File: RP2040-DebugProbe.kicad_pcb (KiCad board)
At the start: 4 copper layers, 59.7 x 31.1 mm, 70 parts, among them J1 CONN_MCU_JTAG, J10 CONN_USB, J2 CONN_MCU_UART, J3 CONN_DBG_COMB, J4 CONN_3V3_JUMPER, J7 CONN_DBG_JTAG, SW1 BOOTSEL, U1 W25Q128JVS, U2 RP2040, U3 74AUP1T17, U4 W25Q128JVEIQ, U5 AMS1117-3.3, U6 74AUP1T17, Y1 12MHz

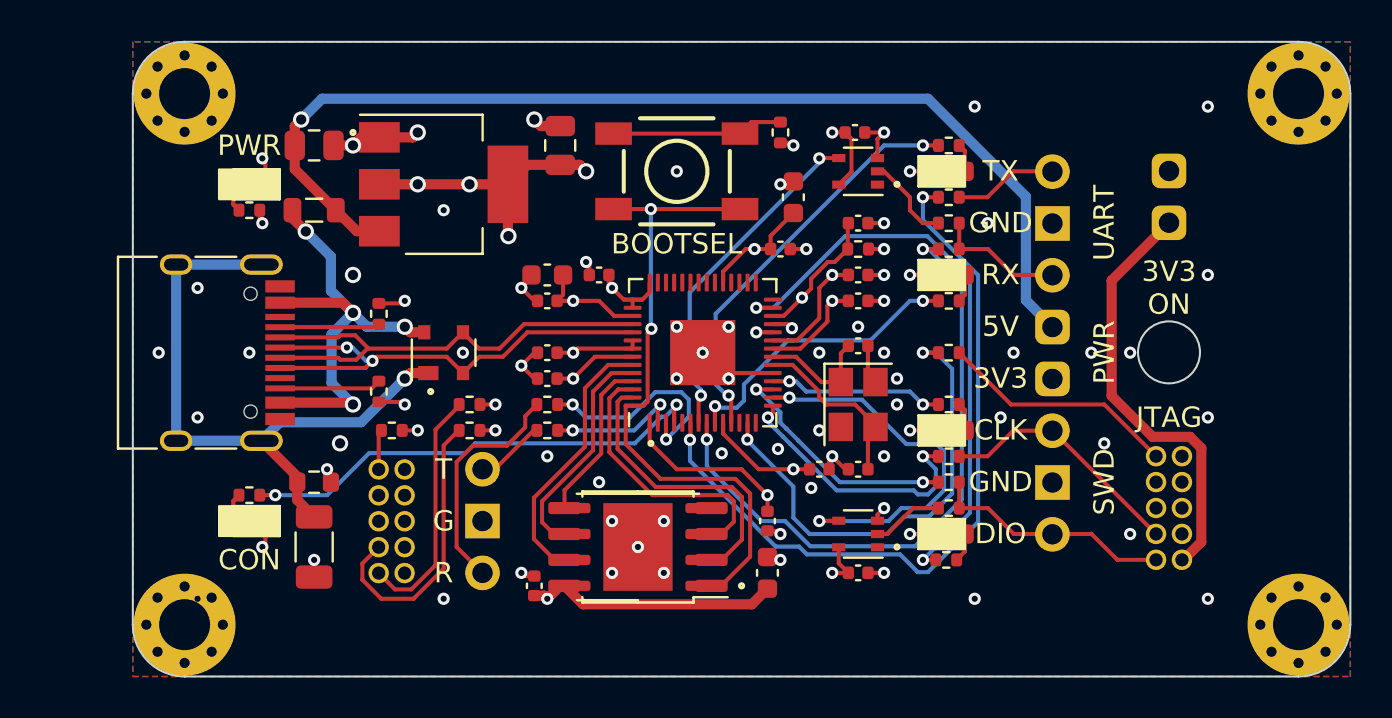
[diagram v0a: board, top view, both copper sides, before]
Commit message: tinyprogrammer
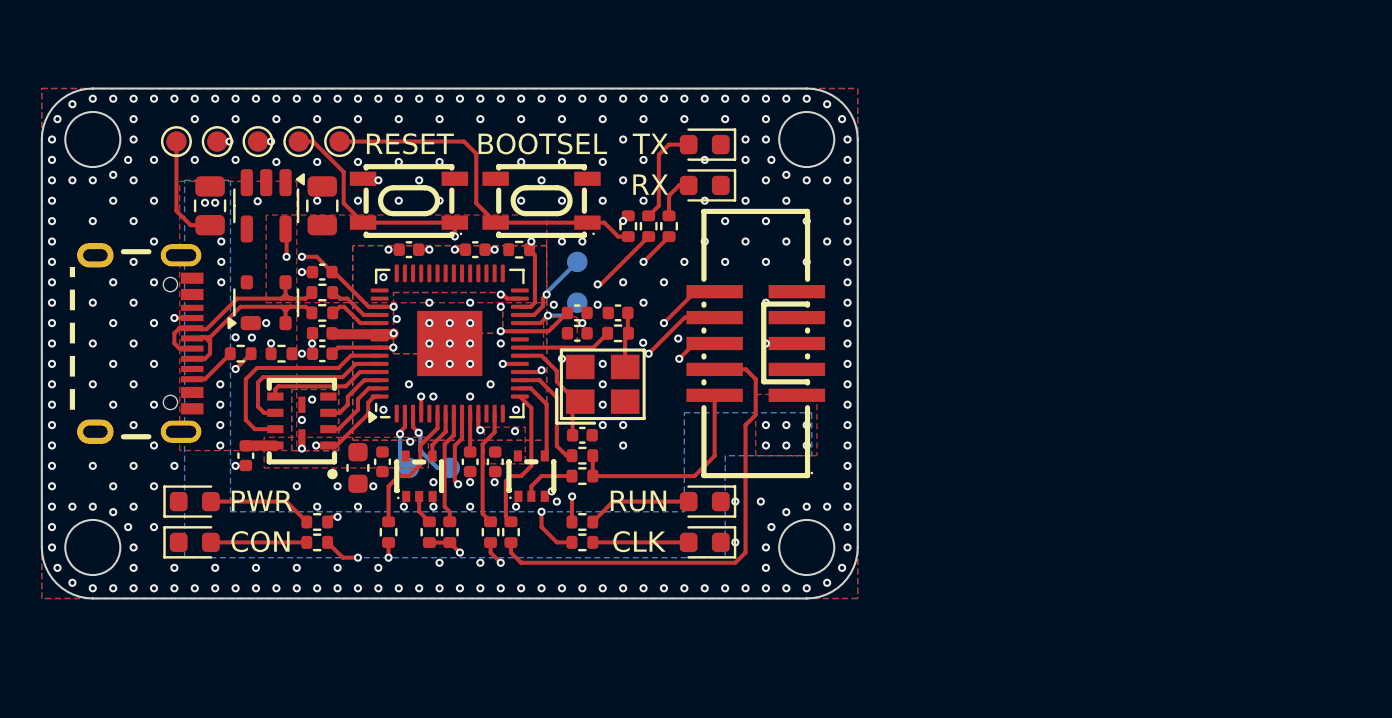
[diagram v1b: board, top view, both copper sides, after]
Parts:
- removed C1, C5: 2.2uF, Capacitor_SMD:C_0603_1608Metric
- removed C12, C13: 100nF, Capacitor_SMD:C_0402_1005Metric
- removed C21: 4.7nF 1kV, Capacitor_SMD:C_1206_3216Metric
- removed FB2: 100@100MHz, Inductor_SMD:L_0805_2012Metric
- removed H1, H2, H3, H4: MountingHole_Pad, MountingHole:MountingHole_2.5mm_Pad_Via
- removed J1: CONN_MCU_JTAG, Connector_PinHeader_1.27mm:PinHeader_2x05_P1.27mm_Vertical
- removed J2: CONN_MCU_UART, Connector_PinHeader_2.54mm:PinHeader_1x03_P2.54mm_Vertical
- removed J3: CONN_DBG_COMB, Connector_PinHeader_2.54mm:PinHeader_1x08_P2.54mm_Vertical
- removed J4: CONN_3V3_JUMPER, Connector_PinHeader_2.54mm:PinHeader_1x02_P2.54mm_Vertical
- removed J7: CONN_DBG_JTAG, Connector_PinHeader_1.27mm:PinHeader_2x05_P1.27mm_Vertical
- removed R20, R21, R22, R23: 100R, Resistor_SMD:R_0402_1005Metric
- removed R8: 10k, Resistor_SMD:R_0402_1005Metric
- removed SW1: BOOTSEL, PCM_4ms_Switch:Button_Tact_Sqkg
- added R24: 27R, Resistor_SMD:R_0402_1005Metric, F.Cu at (133.8, 106.0)
- added R25: 27R, Resistor_SMD:R_0402_1005Metric, F.Cu at (133.8, 105.0)
- added TP10: TestPoint, TestPoint:TestPoint_Pad_D1.0mm, B.Cu at (146.2, 103.5)
- added TP11: TestPoint, TestPoint:TestPoint_Pad_D1.0mm, B.Cu at (146.2, 105.5)
- added TP13: TestPoint, TestPoint:TestPoint_Pad_D1.0mm, F.Cu at (130.6, 97.6)
- added TP4: TestPoint, TestPoint:TestPoint_Pad_D1.0mm, F.Cu at (126.6, 97.6)
- added TP5: TestPoint, TestPoint:TestPoint_Pad_D1.0mm, F.Cu at (128.6, 97.6)
- added TP6: TestPoint, TestPoint:TestPoint_Pad_D1.0mm, F.Cu at (134.6, 97.6)
- added TP7: TestPoint, TestPoint:TestPoint_Pad_D1.0mm, F.Cu at (132.6, 97.6)
- added TP8: TestPoint, TestPoint:TestPoint_Pad_D1.0mm, B.Cu at (138.0, 113.6)
- added TP9: TestPoint, TestPoint:TestPoint_Pad_D1.0mm, B.Cu at (140.0, 113.6)
- added U7: HX_JN1_27-2X5_TP_H4_9, JLCPCB:IDC-SMD_10P-P1.27-3220-10-0300-00, F.Cu at (155.0, 107.5)
- added U8: TS-1089S-02526, JLCPCB:SW-SMD_4P-L4.2-W3.3-P2.15-LS5.1, F.Cu at (138.0, 100.5)
- C14, C15: value 10uF -> 22uF
- C19, C20: value 12pF -> 15pF
- J10: footprint Connector_USB:USB_C_Receptacle_HRO_TYPE-C-31-M-12 -> JLCPCB:USB-C-SMD_TYPE-C-6PIN-2MD-073
- R12: value 1M -> 1K; footprint Resistor_SMD:R_0603_1608Metric -> Resistor_SMD:R_0402_1005Metric
- R19: value 100R -> 10k
- U1: value W25Q128JVS -> AP2112K-3.3; footprint Package_SO:SOIC-8_5.23x5.23mm_P1.27mm -> Package_TO_SOT_SMD:SOT-23-5
- U3, U6: value 74AUP1T17 -> 74AUP1T17GWH; footprint Package_TO_SOT_SMD:SOT-353_SC-70-5 -> JLCPCB:TSSOP-5_L2.1-W1.3-P0.65-LS2.2-BR
- U4: value W25Q128JVEIQ -> W25Q64JVEIQ; footprint Package_SON:WSON-8-1EP_6x5mm_P1.27mm_EP3.4x4.3mm -> JLCPCB:USON-8_L4.0-W3.0-P0.80-BL_WINBOND_UU
- U5: value AMS1117-3.3 -> TS-1089S-02526; footprint Package_TO_SOT_SMD:SOT-223-3_TabPin2 -> JLCPCB:SW-SMD_4P-L4.2-W3.3-P2.15-LS5.1
- Y1: footprint Crystal:Crystal_SMD_3225-4Pin_3.2x2.5mm -> JLCPCB:CRYSTAL-SMD_4P-L3.2-W2.5-BL
- moved R15 32.0 mm to (137.0, 116.8), turned to 90 degrees
- moved R9 29.6 mm to (139.0, 116.8), turned to 90 degrees
- moved C17 28.2 mm to (136.7, 113.3), turned to -90 degrees
- moved R14 28.1 mm to (140.0, 116.8), turned to 90 degrees
- moved U3 26.2 mm to (138.5, 114.0), turned to -90 degrees
- moved U1 24.7 mm to (131.0, 100.8), turned to -90 degrees
- moved R18 24.1 mm to (142.0, 116.8), turned to 90 degrees
- moved R17 21.8 mm to (143.0, 116.8), turned to 90 degrees
- moved C16 20.7 mm to (135.5, 113.6), turned to -90 degrees
- moved C3 19.6 mm to (141.2, 102.9), turned to 0 degrees
- moved R4 19.2 mm to (146.5, 117.2)
- moved C4 18.2 mm to (138.0, 102.9)
- moved R13 18.0 mm to (146.5, 114.0)
- moved R16 18.0 mm to (146.5, 113.0)
- moved R5 17.9 mm to (146.5, 116.2)
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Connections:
- net Net-(D1-A) renamed /RLED_RX
- net Net-(D4-A) renamed /RLED_TX
- net Net-(D5-A) renamed /RLED_ACT
- net Net-(D6-A) renamed /RLED_CON
- net Net-(D7-A) renamed /RLED_RUN
- C15 pad 1: VUSB -> +5V
- C19 pad 1: XIN -> /XIN
- C20 pad 1: XOUT -> /ROUT
- D3 pad 1: SHIELD -> GND
- D3 pad 2: USB_DP -> USBC_DP
- D3 pad 3: USB_DN -> USBC_DN
- D3 pad 4: VBUS -> +5V
- R10 pad 1: Net-(J10-CC1) -> /CC1
- R11 pad 1: Net-(J10-CC2) -> /CC2
- R12 pad 1: SHIELD -> /XOUT
- R12 pad 2: GND -> /ROUT
- R19 pad 1: MCU_TX -> +3V3
- R19 pad 2: HOST_TX -> /RESET
- R7 pad 1: Net-(R7-Pad1) -> /QSPI_SS
- R7 pad 2: GND -> /BOOTSEL
- U1 pad 1: QSPI_SS -> +5V
- U1 pad 2: QSPI_SD1 -> GND
- U1 pad 3: QSPI_SD2 -> +5V
- U1 pad 4: GND -> unconnected-(U1-NC-Pad4)
- U1 pad 5: QSPI_SD0 -> +3V3
- U2 pad 2: MCU_TX -> /HOST_UART_TX
- U2 pad 20: XIN -> /XIN
- U2 pad 21: XOUT -> /XOUT
- U2 pad 24: MCU_CLK -> /HOST_SWCLK_RX
- U2 pad 25: MCU_DIO -> /HOST_SWDIO_TX
- U2 pad 26: MCU_RESET -> /RESET
- U2 pad 3: MCU_RX -> /HOST_UART_RX
- U2 pad 46: USB_DN -> /USB_DN
- U2 pad 47: USB_DP -> /USB_DP
- U2 pad 51: QSPI_SD3 -> /QSPI_SD3
- U2 pad 52: QSPI_SCLK -> /QSPI_CLK
- U2 pad 53: QSPI_SD0 -> /QSPI_SD0
- U2 pad 54: QSPI_SD2 -> /QSPI_SD2
- U2 pad 55: QSPI_SD1 -> /QSPI_SD1
- U2 pad 56: QSPI_SS -> /QSPI_SS
- U3 pad 1: (no net) -> GND
- U4 pad 1: QSPI_SS -> /QSPI_SS
- U4 pad 2: QSPI_SD1 -> /QSPI_SD1
- U4 pad 3: QSPI_SD2 -> /QSPI_SD2
- U4 pad 5: QSPI_SD0 -> /QSPI_SD0
- U4 pad 6: QSPI_SCLK -> /QSPI_CLK
- U4 pad 7: QSPI_SD3 -> /QSPI_SD3
- U5 pad 1: GND -> /BOOTSEL
- U5 pad 2: +3V3 -> /BOOTSEL
- U5 pad 3: VUSB -> GND
- U6 pad 1: (no net) -> GND
- Y1 pad 1: XOUT -> /XIN
- Y1 pad 3: XIN -> /ROUT
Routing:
- net VUSB: track 52.8 -> 0.00 mm, vias 1 -> 0
- net +3V3: track 66.4 -> 24.3 mm, vias 15 -> 14
- net GND: track 38.3 -> 3.42 mm, vias 76 -> 306
- net QSPI_SS: track 31.5 -> 0.00 mm, vias 2 -> 0
- net SHIELD: track 31.4 -> 0.00 mm, vias 1 -> 0
- net UART_TX: track 37.1 -> 6.59 mm, vias 2 -> 0
- net /QSPI_SS: track 0.00 -> 29.8 mm, vias 0 -> 2
- net MCU_RESET: track 29.0 -> 0.00 mm, vias 2 -> 0
- net UART_RX: track 31.2 -> 5.74 mm, vias 2 -> 0
- net USB_DP: track 23.5 -> 0.00 mm, vias 2 -> 0
- net USB_DN: track 23.4 -> 0.00 mm
- net VBUS: track 22.9 -> 0.00 mm, vias 4 -> 0
- net TARGET_TX: track 5.10 -> 27.7 mm, vias 0 -> 2
- net MCU_CLK: track 22.5 -> 0.00 mm, vias 2 -> 0
- net TARGET_3V3: track 21.0 -> 0.00 mm
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- added copper zone on B.Cu, net +1V1
- added copper zone on F.Cu, net +1V1
- added copper zone on B.Cu, net +3V3
- added copper zone on F.Cu, net +3V3
- added copper zone on B.Cu, net +5V
- added copper zone on F.Cu, net +5V
- added copper zone on In2.Cu, net GND
- removed copper zone on In2.Cu, net +3V3
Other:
- board size 59.7 x 31.1 mm -> 40 x 25 mm
- board text added: "BOOTSEL"
- board text added: "RESET"
- board text added: "RUN"
- board text added: "SWCLK"
- board text added: "SWDIO"
- board text removed: "${TITLE} ${COMPANY} ${COMMENT2}"
- board text removed: "3V3"
- board text removed: "3V3 ON"
- board text removed: "5V"
- board text removed: "DIO"
- board text removed: "G"
- board text removed: "GND"
- board text removed: "JTAG"
- board text removed: "R"
- board text removed: "SWD"
- board text removed: "T"
- board text removed: "UART"
